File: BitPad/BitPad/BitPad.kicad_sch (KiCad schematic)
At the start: 10 parts, among them SW1 SW_Push, SW2 SW_Push, SW3 SW_Push, SW4 SW_Push, SW5 SW_MEC_5E, U1 MOUDLE-SEEEDUINO-XIAO

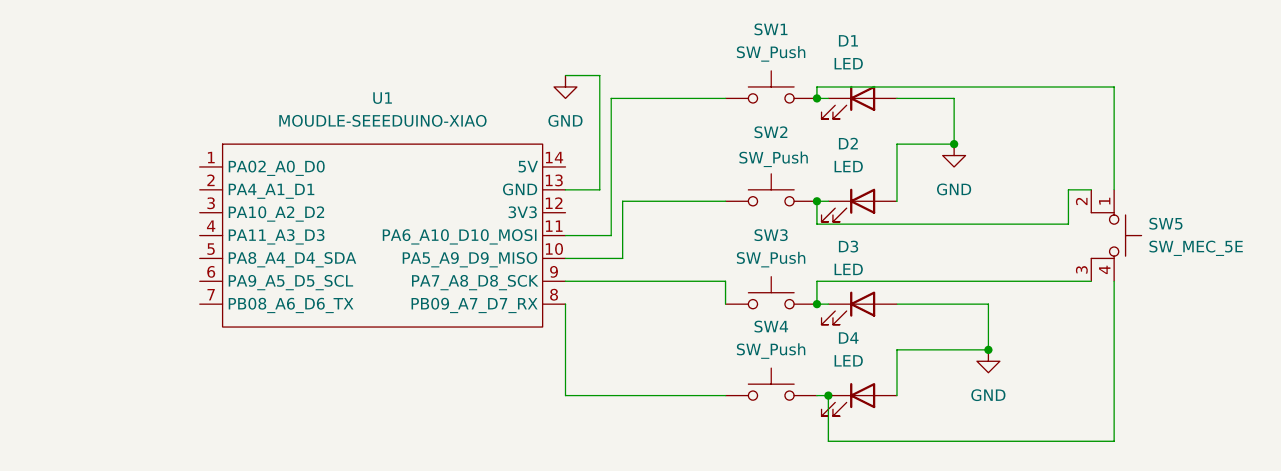
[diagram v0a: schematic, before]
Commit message: updated the kicad files
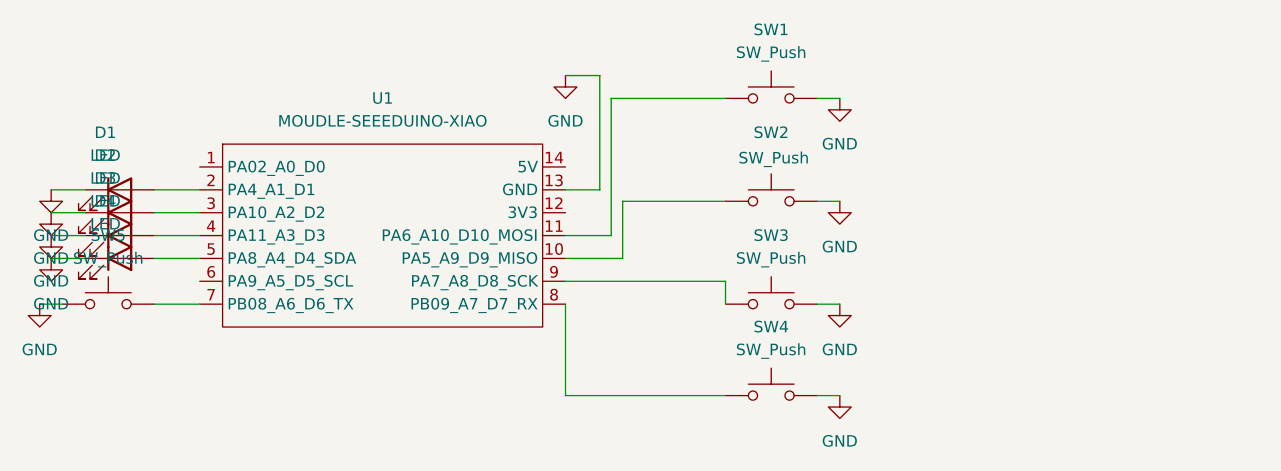
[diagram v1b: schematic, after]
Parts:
- removed SW5: SW_MEC_5E, Button_Switch_Keyboard:SW_Cherry_MX_1.00u_PCB, symbol Switch:SW_MEC_5E
- added SW5: SW_Push, Button_Switch_THT:SW_TH_Tactile_Omron_B3F-100x, symbol Switch:SW_Push
- D1, D2, D3, D4: footprint Diode_SMD:D_SMA -> Diode_SMD:D_0201_0603Metric
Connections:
- net GND: now also D1.1 (K), D2.1 (K), D3.1 (K), D4.1 (K), SW1.2, SW2.2, SW3.2, SW4.2, SW5.1; no longer D1.2 (A), D2.2 (A), D3.2 (A), D4.2 (A)
- net at U1.2 (PA4_A1_D1): now also D1.2 (A)
- net at U1.3 (PA10_A2_D2): now also D2.2 (A)
- net at U1.4 (PA11_A3_D3): now also D3.2 (A)
- net at U1.5 (PA8_A4_D4_SDA): now also D4.2 (A)
- net at U1.7 (PB08_A6_D6_TX): now also SW5.2
